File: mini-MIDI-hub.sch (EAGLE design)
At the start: 59 parts, among them IC1 6N138, IC2 PIC16F1825SO14, IC3 4050D, IC4 REG1117, IC5 REG1117, X1 DIN5PIN, X2 DIN5PIN, X3 DIN5PIN, X4 DIN5PIN, X5 DIN5PIN, X6 DIN5PIN

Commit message: tweakz
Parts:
- renumbered J1 to ICSP
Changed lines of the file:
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@@
 <part name="GND1" library="supply1" deviceset="GND" device=""/>
 <part name="IC2" library="jasons_stuff" deviceset="PIC16F1825" device="SO14"/>
-<part name="J1" library="tag-connect" deviceset="TC2030" device="-MCP-NL"/>
+<part name="ICSP" library="tag-connect" deviceset="TC2030" device="-MCP-NL"/>
 <part name="GND2" library="supply1" deviceset="GND" device=""/>
 <part name="GND3" library="supply1" deviceset="GND" device=""/>
@@
 <instance part="GND1" gate="1" x="317.5" y="33.02"/>
 <instance part="IC2" gate="G$1" x="360.68" y="38.1"/>
-<instance part="J1" gate="G$1" x="414.02" y="43.18"/>
+<instance part="ICSP" gate="G$1" x="414.02" y="43.18"/>
 <instance part="GND2" gate="1" x="15.24" y="33.02"/>
 <instance part="GND3" gate="1" x="22.86" y="33.02"/>
@@
 <segment>
 <pinref part="IC2" gate="G$1" pin="VSS"/>
-<pinref part="J1" gate="G$1" pin="VSS(GND)"/>
+<pinref part="ICSP" gate="G$1" pin="VSS(GND)"/>
 <wire x1="383.54" y1="45.72" x2="386.08" y2="45.72" width="0.1524" layer="91"/>
 <pinref part="C3" gate="G$1" pin="1"/>
@@
 <wire x1="337.82" y1="53.34" x2="398.78" y2="53.34" width="0.1524" layer="91"/>
 <wire x1="398.78" y1="53.34" x2="398.78" y2="50.8" width="0.1524" layer="91"/>
-<pinref part="J1" gate="G$1" pin="VPP/MCLR"/>
+<pinref part="ICSP" gate="G$1" pin="VPP/MCLR"/>
 <wire x1="401.32" y1="50.8" x2="398.78" y2="50.8" width="0.1524" layer="91"/>
 </segment>
@@
 <segment>
 <pinref part="IC2" gate="G$1" pin="RA0/ICSPDAT"/>
-<pinref part="J1" gate="G$1" pin="ICSP_DAT/PGD"/>
+<pinref part="ICSP" gate="G$1" pin="ICSP_DAT/PGD"/>
 <wire x1="383.54" y1="43.18" x2="388.62" y2="43.18" width="0.1524" layer="91"/>
 <wire x1="388.62" y1="43.18" x2="401.32" y2="43.18" width="0.1524" layer="91"/>
@@
 <segment>
 <pinref part="IC2" gate="G$1" pin="RA1/ICPCLK"/>
-<pinref part="J1" gate="G$1" pin="ICSP_CLK/PGC"/>
+<pinref part="ICSP" gate="G$1" pin="ICSP_CLK/PGC"/>
 <wire x1="383.54" y1="40.64" x2="391.16" y2="40.64" width="0.1524" layer="91"/>
 <wire x1="391.16" y1="40.64" x2="401.32" y2="40.64" width="0.1524" layer="91"/>

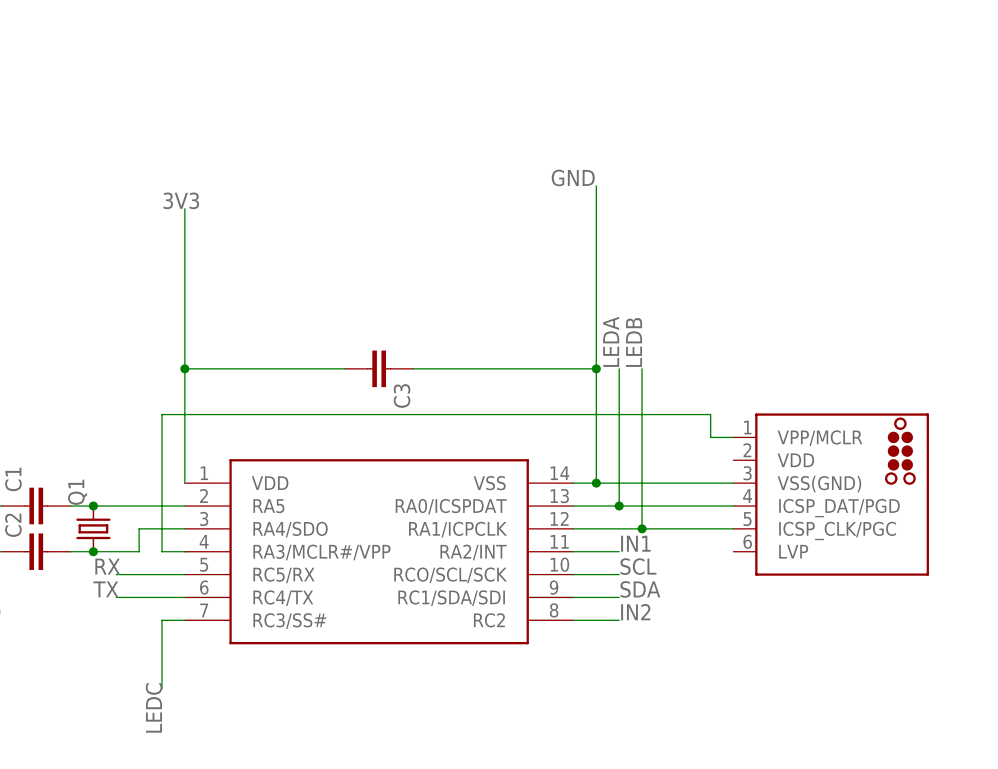
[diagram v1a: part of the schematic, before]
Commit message: tweaks
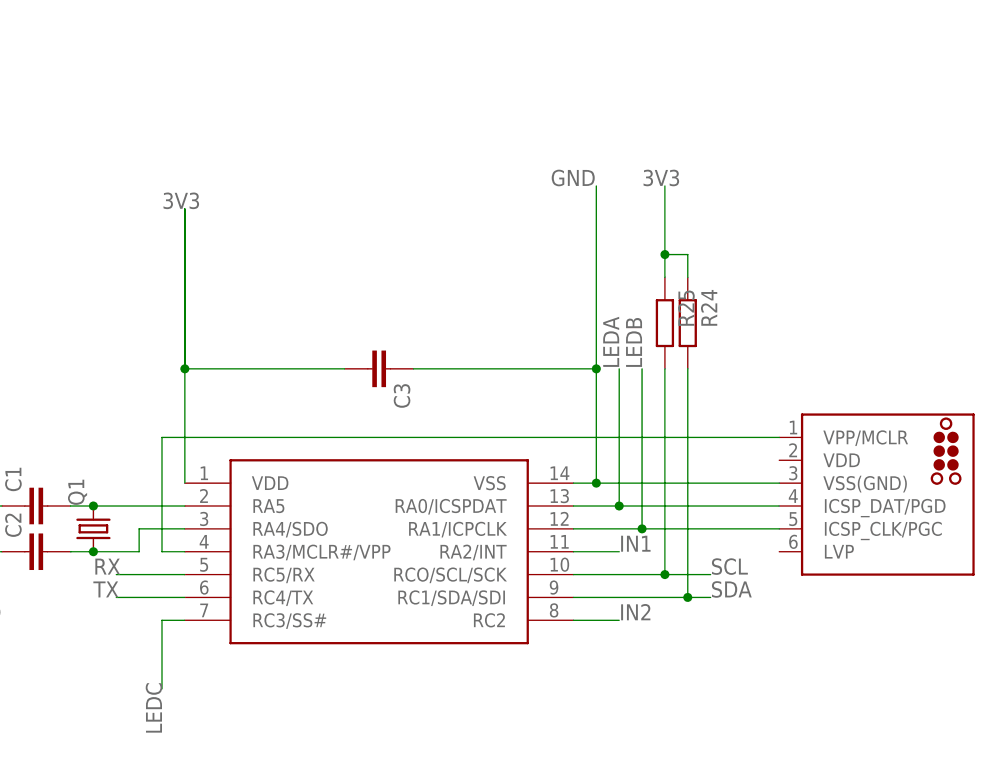
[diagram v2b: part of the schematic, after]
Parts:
- added R24, R25: (no value), rcl:R-EU_R0805
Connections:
- net 3V3: now also R24.1, R25.1
- net SCL: now also R25.2
- net SDA: now also R24.2
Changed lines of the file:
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@@
 <part name="U$3" library="jason_eagle6" deviceset="LED5MM_EDGE" device=""/>
 <part name="U$4" library="jason_eagle6" deviceset="LED5MM_EDGE" device=""/>
+<part name="R25" library="rcl" deviceset="R-EU_" device="R0805"/>
+<part name="R24" library="rcl" deviceset="R-EU_" device="R0805"/>
 </parts>
 <sheets>
@@
 <instance part="GND1" gate="1" x="317.5" y="33.02"/>
 <instance part="IC2" gate="G$1" x="360.68" y="38.1"/>
-<instance part="ICSP" gate="G$1" x="414.02" y="43.18"/>
+<instance part="ICSP" gate="G$1" x="419.1" y="43.18"/>
 <instance part="GND2" gate="1" x="15.24" y="33.02"/>
 <instance part="GND3" gate="1" x="22.86" y="33.02"/>
@@
 <instance part="U$3" gate="G$1" x="17.78" y="-2.54" rot="R270"/>
 <instance part="U$4" gate="G$1" x="22.86" y="-2.54" rot="R270"/>
+<instance part="R25" gate="G$1" x="393.7" y="63.5" rot="R270"/>
+<instance part="R24" gate="G$1" x="396.24" y="63.5" rot="R270"/>
 </instances>
 <busses>
@@
 <wire x1="383.54" y1="45.72" x2="386.08" y2="45.72" width="0.1524" layer="91"/>
 <pinref part="C3" gate="G$1" pin="1"/>
-<wire x1="386.08" y1="45.72" x2="401.32" y2="45.72" width="0.1524" layer="91"/>
+<wire x1="386.08" y1="45.72" x2="406.4" y2="45.72" width="0.1524" layer="91"/>
 <wire x1="365.76" y1="58.42" x2="386.08" y2="58.42" width="0.1524" layer="91"/>
 <wire x1="386.08" y1="58.42" x2="386.08" y2="45.72" width="0.1524" layer="91"/>
@@
 <pinref part="IC2" gate="G$1" pin="RA3/MCLR#/VPP"/>
 <wire x1="340.36" y1="38.1" x2="337.82" y2="38.1" width="0.1524" layer="91"/>
-<wire x1="337.82" y1="38.1" x2="337.82" y2="53.34" width="0.1524" layer="91"/>
-<wire x1="337.82" y1="53.34" x2="398.78" y2="53.34" width="0.1524" layer="91"/>
-<wire x1="398.78" y1="53.34" x2="398.78" y2="50.8" width="0.1524" layer="91"/>
+<wire x1="337.82" y1="38.1" x2="337.82" y2="50.8" width="0.1524" layer="91"/>
+<wire x1="337.82" y1="50.8" x2="406.4" y2="50.8" width="0.1524" layer="91"/>
 <pinref part="ICSP" gate="G$1" pin="VPP/MCLR"/>
-<wire x1="401.32" y1="50.8" x2="398.78" y2="50.8" width="0.1524" layer="91"/>
 </segment>
 </net>
@@
 <segment>
 <pinref part="IC2" gate="G$1" pin="RCO/SCL/SCK"/>
-<wire x1="383.54" y1="35.56" x2="388.62" y2="35.56" width="0.1524" layer="91"/>
-<label x="388.62" y="35.56" size="1.778" layer="95"/>
+<wire x1="383.54" y1="35.56" x2="393.7" y2="35.56" width="0.1524" layer="91"/>
+<label x="398.78" y="35.56" size="1.778" layer="95"/>
+<pinref part="R25" gate="G$1" pin="2"/>
+<wire x1="393.7" y1="35.56" x2="398.78" y2="35.56" width="0.1524" layer="91"/>
+<wire x1="393.7" y1="58.42" x2="393.7" y2="35.56" width="0.1524" layer="91"/>
+<junction x="393.7" y="35.56"/>
 </segment>
 <segment>
@@
 <segment>
 <pinref part="IC2" gate="G$1" pin="RC1/SDA/SDI"/>
-<wire x1="383.54" y1="33.02" x2="388.62" y2="33.02" width="0.1524" layer="91"/>
-<label x="388.62" y="33.02" size="1.778" layer="95"/>
+<wire x1="383.54" y1="33.02" x2="396.24" y2="33.02" width="0.1524" layer="91"/>
+<label x="398.78" y="33.02" size="1.778" layer="95"/>
+<pinref part="R24" gate="G$1" pin="2"/>
+<wire x1="396.24" y1="33.02" x2="398.78" y2="33.02" width="0.1524" layer="91"/>
+<wire x1="396.24" y1="58.42" x2="396.24" y2="33.02" width="0.1524" layer="91"/>
+<junction x="396.24" y="33.02"/>
 </segment>
 <segment>
@@
 <pinref part="ICSP" gate="G$1" pin="ICSP_DAT/PGD"/>
 <wire x1="383.54" y1="43.18" x2="388.62" y2="43.18" width="0.1524" layer="91"/>
-<wire x1="388.62" y1="43.18" x2="401.32" y2="43.18" width="0.1524" layer="91"/>
+<wire x1="388.62" y1="43.18" x2="406.4" y2="43.18" width="0.1524" layer="91"/>
 <wire x1="388.62" y1="43.18" x2="388.62" y2="58.42" width="0.1524" layer="91"/>
 <junction x="388.62" y="43.18"/>
@@
 <pinref part="ICSP" gate="G$1" pin="ICSP_CLK/PGC"/>
 <wire x1="383.54" y1="40.64" x2="391.16" y2="40.64" width="0.1524" layer="91"/>
-<wire x1="391.16" y1="40.64" x2="401.32" y2="40.64" width="0.1524" layer="91"/>
+<wire x1="391.16" y1="40.64" x2="406.4" y2="40.64" width="0.1524" layer="91"/>
 <wire x1="391.16" y1="40.64" x2="391.16" y2="58.42" width="0.1524" layer="91"/>
 <junction x="391.16" y="40.64"/>
@@
 <junction x="340.36" y="58.42"/>
 <label x="337.82" y="76.2" size="1.778" layer="95"/>
+<wire x1="340.36" y1="58.42" x2="340.36" y2="76.2" width="0.1524" layer="91"/>
 </segment>
 <segment>
@@
 <label x="228.6" y="116.84" size="1.778" layer="95"/>
 </segment>
-</net>
+<segment>
+<pinref part="R25" gate="G$1" pin="1"/>
+<wire x1="393.7" y1="68.58" x2="393.7" y2="71.12" width="0.1524" layer="91"/>
+<pinref part="R24" gate="G$1" pin="1"/>
+<wire x1="393.7" y1="71.12" x2="396.24" y2="71.12" width="0.1524" layer="91"/>
+<wire x1="396.24" y1="71.12" x2="396.24" y2="68.58" width="0.1524" layer="91"/>
+<wire x1="393.7" y1="71.12" x2="393.7" y2="78.74" width="0.1524" layer="91"/>
+<junction x="393.7" y="71.12"/>
+<label x="391.16" y="78.74" size="1.778" layer="95"/>
+</segment>
+</net>
